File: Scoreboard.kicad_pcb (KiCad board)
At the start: 2 copper layers, 140.5 x 64.5 mm, 237 parts, among them J1 TC2050-IDC-NL, J2 USB-C_Port, J3 TP4057, Q5 HL-2302V, Q6 HL-2302V, Q7 HL-2302V, SW1 SW_Push, SW2 SW_Push, SW3 SW_Push, U1 BC833M, U2 DW01A, U3 IS31FL3729

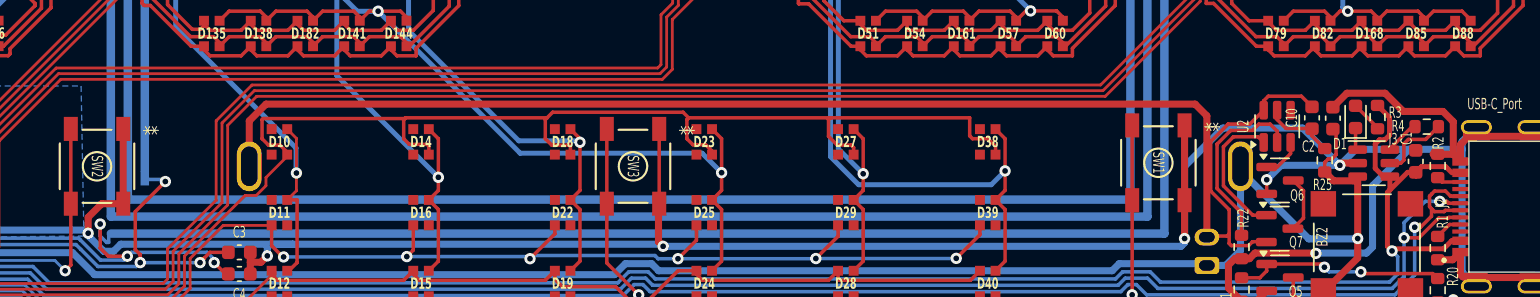
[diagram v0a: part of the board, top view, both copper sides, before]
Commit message: Fixed missing ground connection
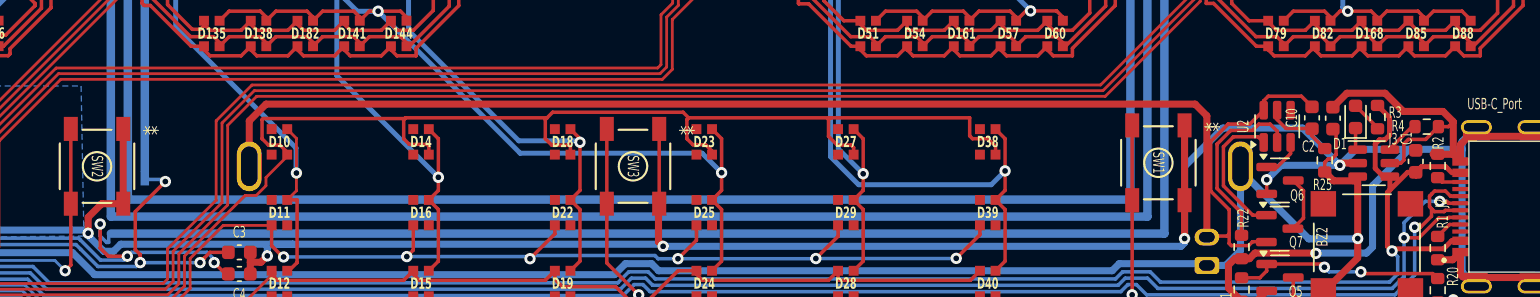
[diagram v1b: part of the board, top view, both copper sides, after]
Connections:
- J3 pad 5: Net-(J3-STDBY) -> GND
- R4 pad 2: Net-(J3-STDBY) -> GND
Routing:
- net GND: track 330.8 -> 337.1 mm
- net Net-(J3-STDBY): track 5.17 -> 0.00 mm
